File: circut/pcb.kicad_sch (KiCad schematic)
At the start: 17 parts, among them J1 GY-302, J2 LD2410B, J3 USB_C_Receptacle_USB2.0, Q1 S8050, U1 AMS1117-3.3, U2 HDC1080, U3 ESP32-S3-WROOM-1

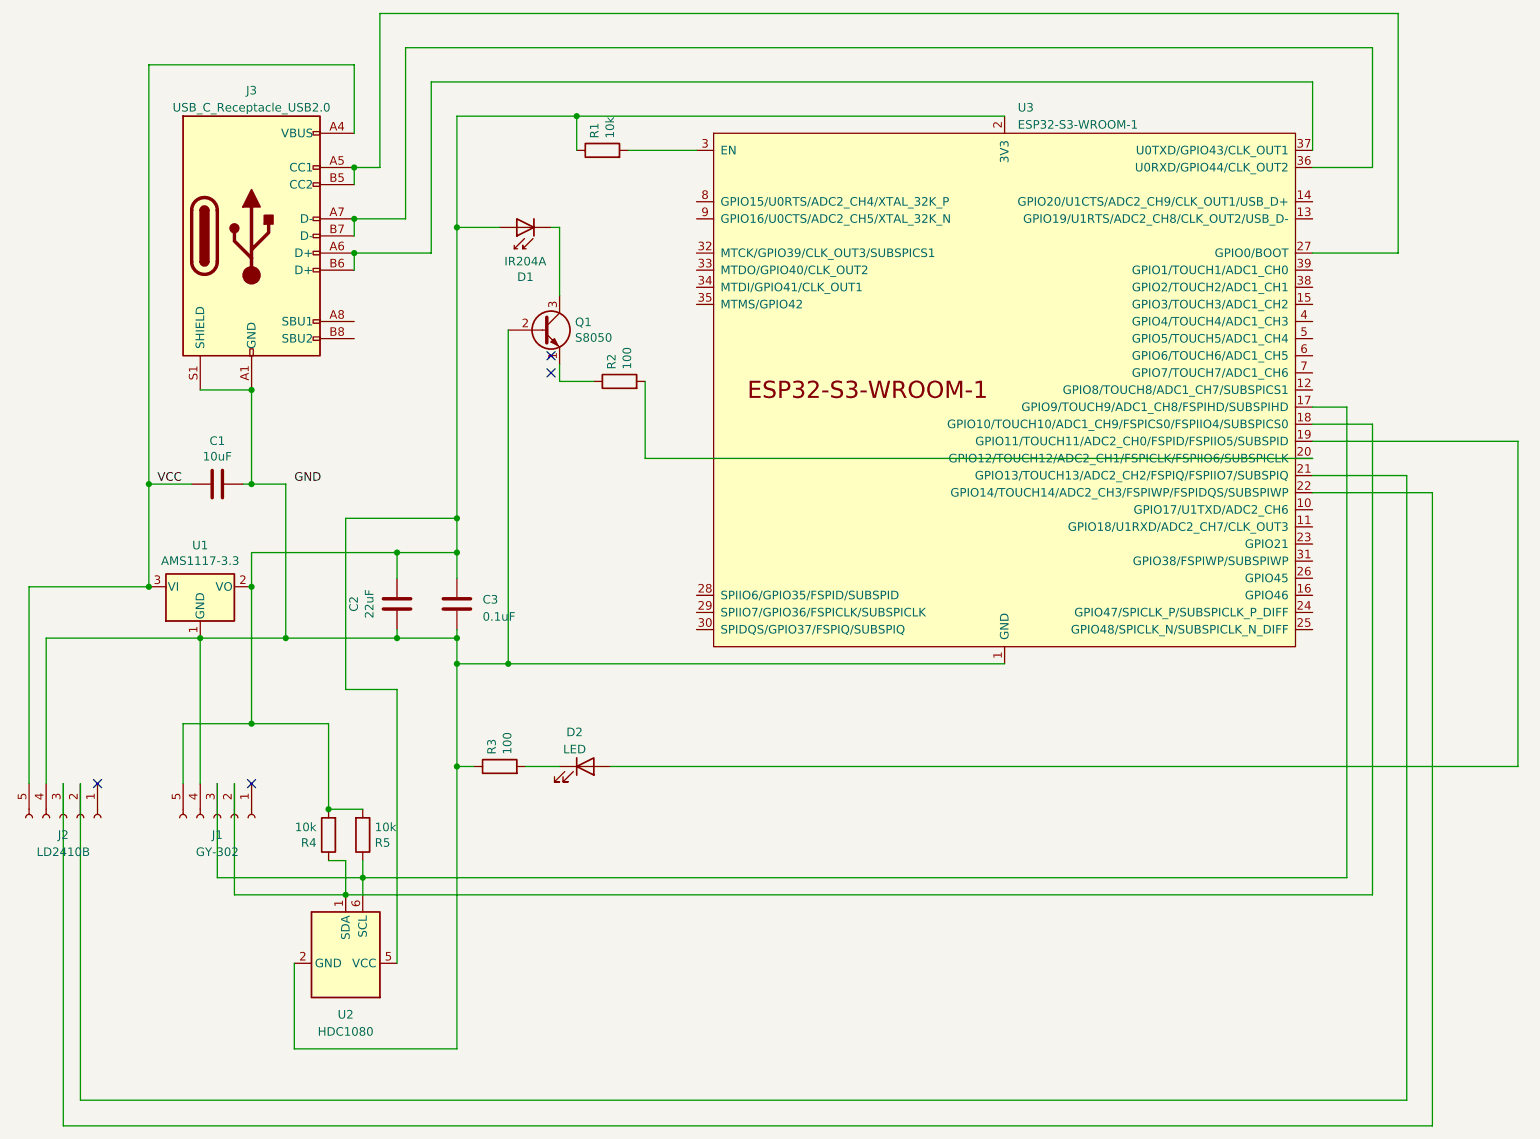
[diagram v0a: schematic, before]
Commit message: optimize pcb layout
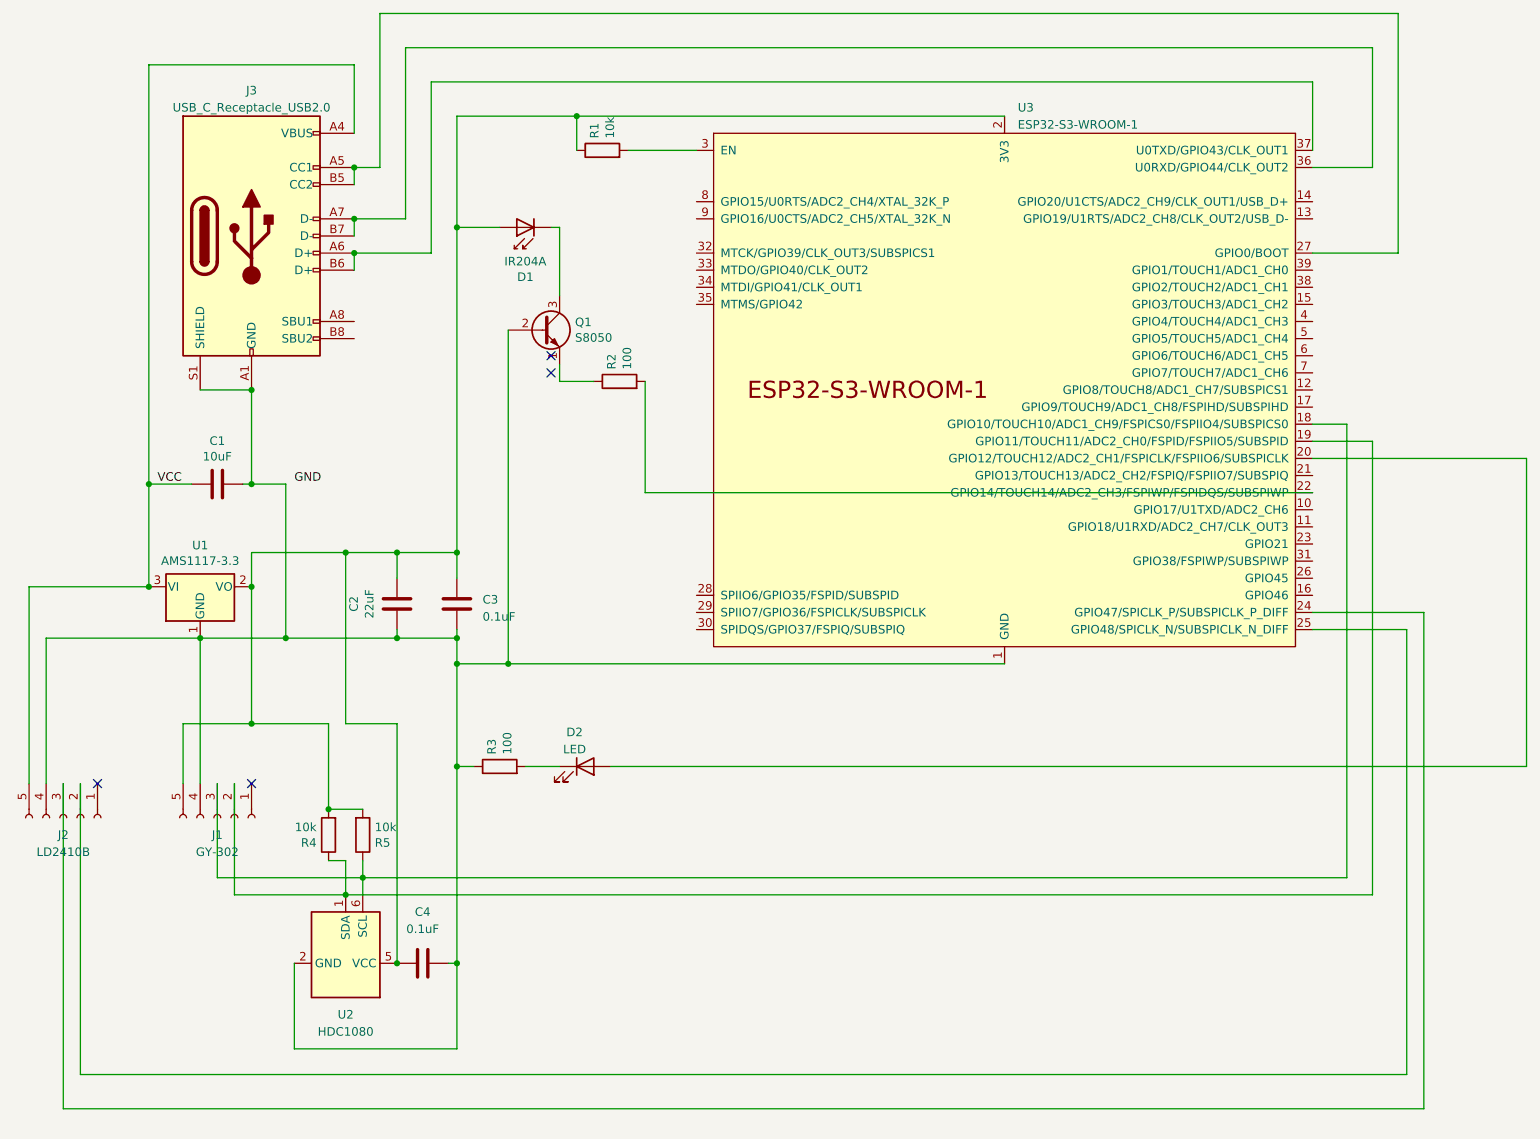
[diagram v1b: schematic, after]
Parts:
- added C4: 0.1uF, Capacitor_SMD:C_0805_2012Metric, symbol Device:C
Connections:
- net at C2.1, C3.1, D1.2 (A)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: now also C4.1
- net at C1.1, C2.2, C3.2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: now also C4.2
- net at J1.2 (Pin_2), R4.1, U2.1 (SDA): now also U3.19 (GPIO11/TOUCH11/ADC2_CH0/FSPID/FSPIIO5/SUBSPID); no longer U3.18 (GPIO10/TOUCH10/ADC1_CH9/FSPICS0/FSPIIO4/SUBSPICS0)
- net at R2.2: now also U3.22 (GPIO14/TOUCH14/ADC2_CH3/FSPIWP/FSPIDQS/SUBSPIWP); no longer U3.20 (GPIO12/TOUCH12/ADC2_CH1/FSPICLK/FSPIIO6/SUBSPICLK)
- net at J2.2 (Pin_2): now also U3.25 (GPIO48/SPICLK_N/SUBSPICLK_N_DIFF); no longer U3.21 (GPIO13/TOUCH13/ADC2_CH2/FSPIQ/FSPIIO7/SUBSPIQ)
- net at J2.3 (Pin_3): now also U3.24 (GPIO47/SPICLK_P/SUBSPICLK_P_DIFF); no longer U3.22 (GPIO14/TOUCH14/ADC2_CH3/FSPIWP/FSPIDQS/SUBSPIWP)
- net at J1.3 (Pin_3), R5.1, U2.6 (SCL): now also U3.18 (GPIO10/TOUCH10/ADC1_CH9/FSPICS0/FSPIIO4/SUBSPICS0); no longer U3.17 (GPIO9/TOUCH9/ADC1_CH8/FSPIHD/SUBSPIHD)
- net at D2.2 (A): now also U3.20 (GPIO12/TOUCH12/ADC2_CH1/FSPICLK/FSPIIO6/SUBSPICLK); no longer U3.19 (GPIO11/TOUCH11/ADC2_CH0/FSPID/FSPIIO5/SUBSPID)
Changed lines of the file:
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@@
   (junction (at 95.25 110.49) (diameter 0) (color 0 0 0 0)
   )
+  (junction (at 95.25 171.45) (diameter 0) (color 0 0 0 0)
+  )
   (junction (at 85.09 148.59) (diameter 0) (color 0 0 0 0)
   )
@@
   (junction (at 73.66 86.36) (diameter 0) (color 0 0 0 0)
   )
-  (junction (at 104.14 105.41) (diameter 0) (color 0 0 0 0)
+  (junction (at 104.14 171.45) (diameter 0) (color 0 0 0 0)
+  )
+  (junction (at 87.63 110.49) (diameter 0) (color 0 0 0 0)
   )
   (junction (at 87.63 161.29) (diameter 0) (color 0 0 0 0)
@@
     (stroke (width 0) (type default))
   )
-  (wire (pts (xy 104.14 142.24) (xy 104.14 184.15))
-    (stroke (width 0) (type default))
-  )
-  (wire (pts (xy 95.25 130.81) (xy 87.63 130.81))
-    (stroke (width 0) (type default))
-  )
-  (wire (pts (xy 95.25 171.45) (xy 95.25 130.81))
+  (wire (pts (xy 104.14 142.24) (xy 104.14 171.45))
+    (stroke (width 0) (type default))
+  )
+  (wire (pts (xy 95.25 135.89) (xy 87.63 135.89))
+    (stroke (width 0) (type default))
+  )
+  (wire (pts (xy 95.25 171.45) (xy 95.25 135.89))
     (stroke (width 0) (type default))
   )
@@
     (stroke (width 0) (type default))
   )
+  (wire (pts (xy 45.72 193.04) (xy 247.65 193.04))
+    (stroke (width 0) (type default))
+  )
   (wire (pts (xy 73.66 135.89) (xy 73.66 115.57))
     (stroke (width 0) (type default))
@@
     (stroke (width 0) (type default))
   )
-  (wire (pts (xy 231.14 91.44) (xy 240.03 91.44))
-    (stroke (width 0) (type default))
-  )
-  (wire (pts (xy 132.08 96.52) (xy 231.14 96.52))
-    (stroke (width 0) (type default))
-  )
   (wire (pts (xy 231.14 40.64) (xy 231.14 50.8))
     (stroke (width 0) (type default))
@@
     (stroke (width 0) (type default))
   )
+  (wire (pts (xy 236.22 158.75) (xy 236.22 91.44))
+    (stroke (width 0) (type default))
+  )
   (wire (pts (xy 88.9 66.04) (xy 88.9 68.58))
     (stroke (width 0) (type default))
   )
+  (wire (pts (xy 87.63 161.29) (xy 240.03 161.29))
+    (stroke (width 0) (type default))
+  )
   (wire (pts (xy 71.12 144.78) (xy 71.12 161.29))
     (stroke (width 0) (type default))
@@
     (stroke (width 0) (type default))
   )
+  (wire (pts (xy 231.14 121.92) (xy 245.11 121.92))
+    (stroke (width 0) (type default))
+  )
   (wire (pts (xy 58.42 38.1) (xy 58.42 100.33))
     (stroke (width 0) (type default))
   )
+  (wire (pts (xy 231.14 96.52) (xy 262.89 96.52))
+    (stroke (width 0) (type default))
+  )
   (wire (pts (xy 104.14 127) (xy 111.76 127))
     (stroke (width 0) (type default))
   )
+  (wire (pts (xy 240.03 161.29) (xy 240.03 93.98))
+    (stroke (width 0) (type default))
+  )
   (wire (pts (xy 104.14 62.23) (xy 104.14 45.72))
     (stroke (width 0) (type default))
   )
+  (wire (pts (xy 236.22 91.44) (xy 231.14 91.44))
+    (stroke (width 0) (type default))
+  )
+  (wire (pts (xy 231.14 93.98) (xy 240.03 93.98))
+    (stroke (width 0) (type default))
+  )
   (wire (pts (xy 119.38 82.55) (xy 119.38 85.09))
     (stroke (width 0) (type default))
@@
     (stroke (width 0) (type default))
   )
-  (wire (pts (xy 248.92 101.6) (xy 248.92 195.58))
+  (wire (pts (xy 247.65 119.38) (xy 247.65 193.04))
     (stroke (width 0) (type default))
   )
@@
     (stroke (width 0) (type default))
   )
-  (wire (pts (xy 87.63 130.81) (xy 87.63 105.41))
+  (wire (pts (xy 87.63 135.89) (xy 87.63 110.49))
     (stroke (width 0) (type default))
   )
@@
     (stroke (width 0) (type default))
   )
-  (wire (pts (xy 127 142.24) (xy 261.62 142.24))
-    (stroke (width 0) (type default))
-  )
-  (wire (pts (xy 87.63 161.29) (xy 240.03 161.29))
-    (stroke (width 0) (type default))
-  )
   (wire (pts (xy 95.25 123.19) (xy 95.25 121.92))
     (stroke (width 0) (type default))
   )
-  (wire (pts (xy 261.62 93.98) (xy 261.62 142.24))
+  (wire (pts (xy 262.89 96.52) (xy 262.89 142.24))
     (stroke (width 0) (type default))
   )
@@
     (stroke (width 0) (type default))
   )
-  (wire (pts (xy 236.22 88.9) (xy 231.14 88.9))
+  (wire (pts (xy 102.87 171.45) (xy 104.14 171.45))
     (stroke (width 0) (type default))
   )
@@
     (stroke (width 0) (type default))
   )
-  (wire (pts (xy 45.72 195.58) (xy 248.92 195.58))
+  (wire (pts (xy 104.14 171.45) (xy 104.14 184.15))
     (stroke (width 0) (type default))
   )
@@
     (stroke (width 0) (type default))
   )
-  (wire (pts (xy 48.26 191.77) (xy 48.26 144.78))
-    (stroke (width 0) (type default))
-  )
-  (wire (pts (xy 104.14 105.41) (xy 104.14 62.23))
+  (wire (pts (xy 48.26 187.96) (xy 48.26 144.78))
     (stroke (width 0) (type default))
   )
@@
     (stroke (width 0) (type default))
   )
-  (wire (pts (xy 104.14 110.49) (xy 104.14 105.41))
-    (stroke (width 0) (type default))
-  )
-  (wire (pts (xy 87.63 105.41) (xy 104.14 105.41))
+  (wire (pts (xy 104.14 62.23) (xy 104.14 110.49))
     (stroke (width 0) (type default))
   )
@@
     (stroke (width 0) (type default))
   )
-  (wire (pts (xy 236.22 88.9) (xy 236.22 158.75))
-    (stroke (width 0) (type default))
-  )
   (wire (pts (xy 78.74 100.33) (xy 78.74 123.19))
     (stroke (width 0) (type default))
@@
     (stroke (width 0) (type default))
   )
-  (wire (pts (xy 231.14 93.98) (xy 261.62 93.98))
+  (wire (pts (xy 45.72 144.78) (xy 45.72 193.04))
     (stroke (width 0) (type default))
   )
@@
     (stroke (width 0) (type default))
   )
-  (wire (pts (xy 45.72 144.78) (xy 45.72 195.58))
-    (stroke (width 0) (type default))
-  )
-  (wire (pts (xy 132.08 85.09) (xy 132.08 96.52))
+  (wire (pts (xy 132.08 85.09) (xy 132.08 101.6))
     (stroke (width 0) (type default))
   )
@@
     (stroke (width 0) (type default))
   )
-  (wire (pts (xy 240.03 91.44) (xy 240.03 161.29))
-    (stroke (width 0) (type default))
-  )
   (wire (pts (xy 88.9 60.96) (xy 88.9 63.5))
     (stroke (width 0) (type default))
@@
     (stroke (width 0) (type default))
   )
+  (wire (pts (xy 87.63 110.49) (xy 95.25 110.49))
+    (stroke (width 0) (type default))
+  )
   (wire (pts (xy 63.5 135.89) (xy 73.66 135.89))
     (stroke (width 0) (type default))
   )
-  (wire (pts (xy 231.14 101.6) (xy 248.92 101.6))
-    (stroke (width 0) (type default))
-  )
   (wire (pts (xy 104.14 62.23) (xy 110.49 62.23))
     (stroke (width 0) (type default))
   )
-  (wire (pts (xy 245.11 191.77) (xy 48.26 191.77))
+  (wire (pts (xy 245.11 187.96) (xy 48.26 187.96))
     (stroke (width 0) (type default))
   )
@@
     (stroke (width 0) (type default))
   )
-  (wire (pts (xy 231.14 99.06) (xy 245.11 99.06))
+  (wire (pts (xy 127 142.24) (xy 262.89 142.24))
     (stroke (width 0) (type default))
   )
@@
     (stroke (width 0) (type default))
   )
-  (wire (pts (xy 73.66 110.49) (xy 95.25 110.49))
+  (wire (pts (xy 231.14 119.38) (xy 247.65 119.38))
+    (stroke (width 0) (type default))
+  )
+  (wire (pts (xy 73.66 110.49) (xy 87.63 110.49))
     (stroke (width 0) (type default))
   )
@@
     (stroke (width 0) (type default))
   )
-  (wire (pts (xy 245.11 99.06) (xy 245.11 191.77))
+  (wire (pts (xy 245.11 121.92) (xy 245.11 187.96))
     (stroke (width 0) (type default))
   )
@@
   )
   (wire (pts (xy 85.09 148.59) (xy 85.09 135.89))
+    (stroke (width 0) (type default))
+  )
+  (wire (pts (xy 132.08 101.6) (xy 231.14 101.6))
     (stroke (width 0) (type default))
   )
@@
         )
       )
+    )
+  )
+  (symbol (lib_id "Device:C") (at 99.06 171.45 90) (unit 1)
+    (in_bom yes) (on_board yes) (dnp no) (fields_autoplaced)
+    (property "Reference" "C4" (at 99.06 163.83 90)
+      (effects (font (size 1.27 1.27)))
+    )
+    (property "Value" "0.1uF" (at 99.06 166.37 90)
+      (effects (font (size 1.27 1.27)))
+    )
+    (property "Footprint" "Capacitor_SMD:C_0805_2012Metric" (at 102.87 170.4848 0)
+      (effects (font (size 1.27 1.27)) hide)
+    )
+    (property "Datasheet" "~" (at 99.06 171.45 0)
+      (effects (font (size 1.27 1.27)) hide)
+    )
+    (pin "1")
+    (pin "2")
+    (instances
+      (project "pcb"
+        (path "/df68c26a-03b5-4466-aecf-ba34b7dce6b7"
+          (reference "C4") (unit 1)
+        )
+      )
